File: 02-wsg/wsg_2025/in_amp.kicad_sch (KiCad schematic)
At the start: 2 parts, among them U4 INA827AIDGK

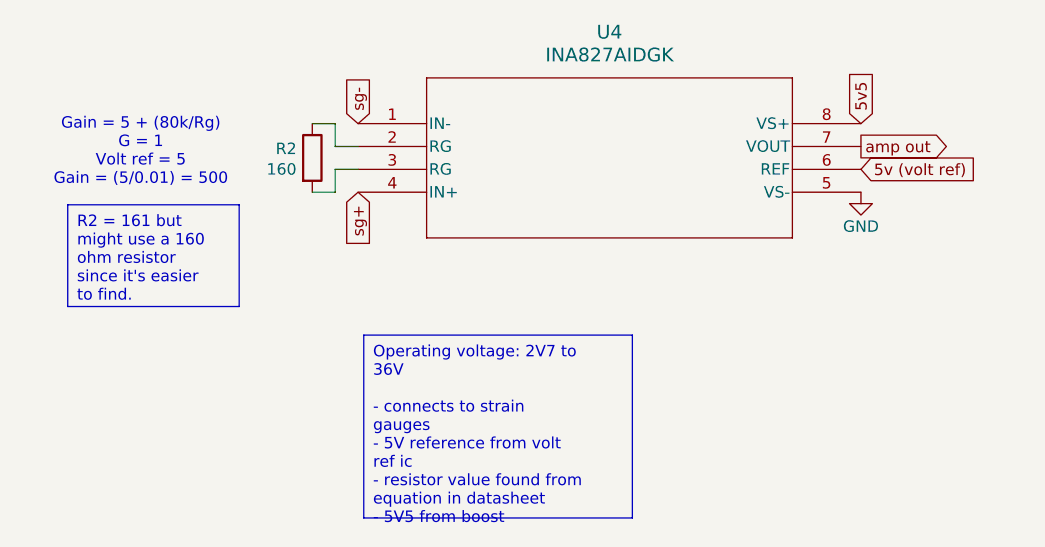
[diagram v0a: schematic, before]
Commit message: new wsg schem - not complete
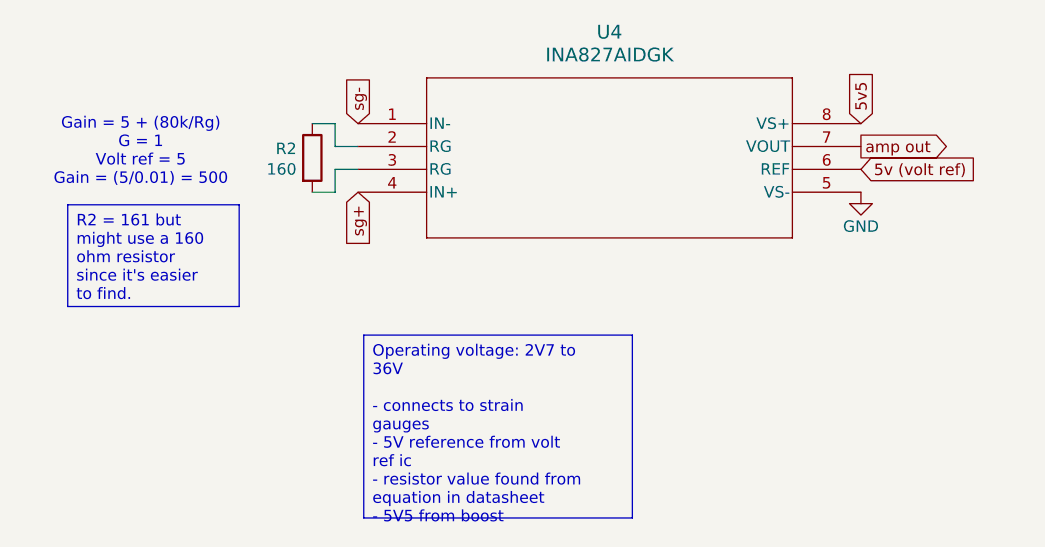
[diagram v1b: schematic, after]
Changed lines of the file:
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@@
 (kicad_sch
-	(version 20231120)
+	(version 20250114)
 	(generator "eeschema")
-	(generator_version "8.0")
+	(generator_version "9.0")
 	(paper "A4")
+	(text "Gain = 5 + (80k/Rg)\nG = 1\nVolt ref = 5\nGain = (5/0.01) = 500"
+		(exclude_from_sim no)
+		(at 67.31 61.595 0)
+		(effects
+			(font
+				(size 1.27 1.27)
+			)
+		)
+	)
+	(text_box "Operating voltage: 2V7 to 36V\n\n- connects to strain gauges\n- 5V reference from volt ref ic\n- resistor value found from equation in datasheet\n- 5V5 from boost"
+		(exclude_from_sim no)
+		(at 92.075 81.915 0)
+		(size 29.845 20.32)
+		(margins 0.9525 0.9525 0.9525 0.9525)
+		(stroke
+			(width 0)
+			(type default)
+		)
+		(fill
+			(type none)
+		)
+		(effects
+			(font
+				(size 1.27 1.27)
+			)
+			(justify left top)
+		)
+	)
+	(text_box "R2 = 161 but might use a 160 ohm resistor since it's easier to find."
+		(exclude_from_sim no)
+		(at 59.182 67.437 0)
+		(size 19.05 11.303)
+		(margins 0.9525 0.9525 0.9525 0.9525)
+		(stroke
+			(width 0)
+			(type default)
+		)
+		(fill
+			(type none)
+		)
+		(effects
+			(font
+				(size 1.27 1.27)
+			)
+			(justify left top)
+		)
+	)
 	(wire
 		(pts
@@
 		)
 	)
-	(text_box "Operating voltage: 2V7 to 36V\n\n- connects to strain gauges\n- 5V reference from volt ref ic\n- resistor value found from equation in datasheet\n- 5V5 from boost"
-		(exclude_from_sim no)
-		(at 92.075 81.915 0)
-		(size 29.845 20.32)
-		(stroke
-			(width 0)
-			(type default)
-		)
-		(fill
-			(type none)
-		)
-		(effects
-			(font
-				(size 1.27 1.27)
-			)
-			(justify left top)
-		)
-	)
-	(text_box "R2 = 161 but might use a 160 ohm resistor since it's easier to find."
-		(exclude_from_sim no)
-		(at 59.182 67.437 0)
-		(size 19.05 11.303)
-		(stroke
-			(width 0)
-			(type default)
-		)
-		(fill
-			(type none)
-		)
-		(effects
-			(font
-				(size 1.27 1.27)
-			)
-			(justify left top)
-		)
-	)
-	(text "Gain = 5 + (80k/Rg)\nG = 1\nVolt ref = 5\nGain = (5/0.01) = 500"
-		(exclude_from_sim no)
-		(at 67.31 61.595 0)
-		(effects
-			(font
-				(size 1.27 1.27)
-			)
-		)
-	)
